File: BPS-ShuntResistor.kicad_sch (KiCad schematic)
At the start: 15 parts, among them J3 Amp_Conn, SW1 SW_DPST

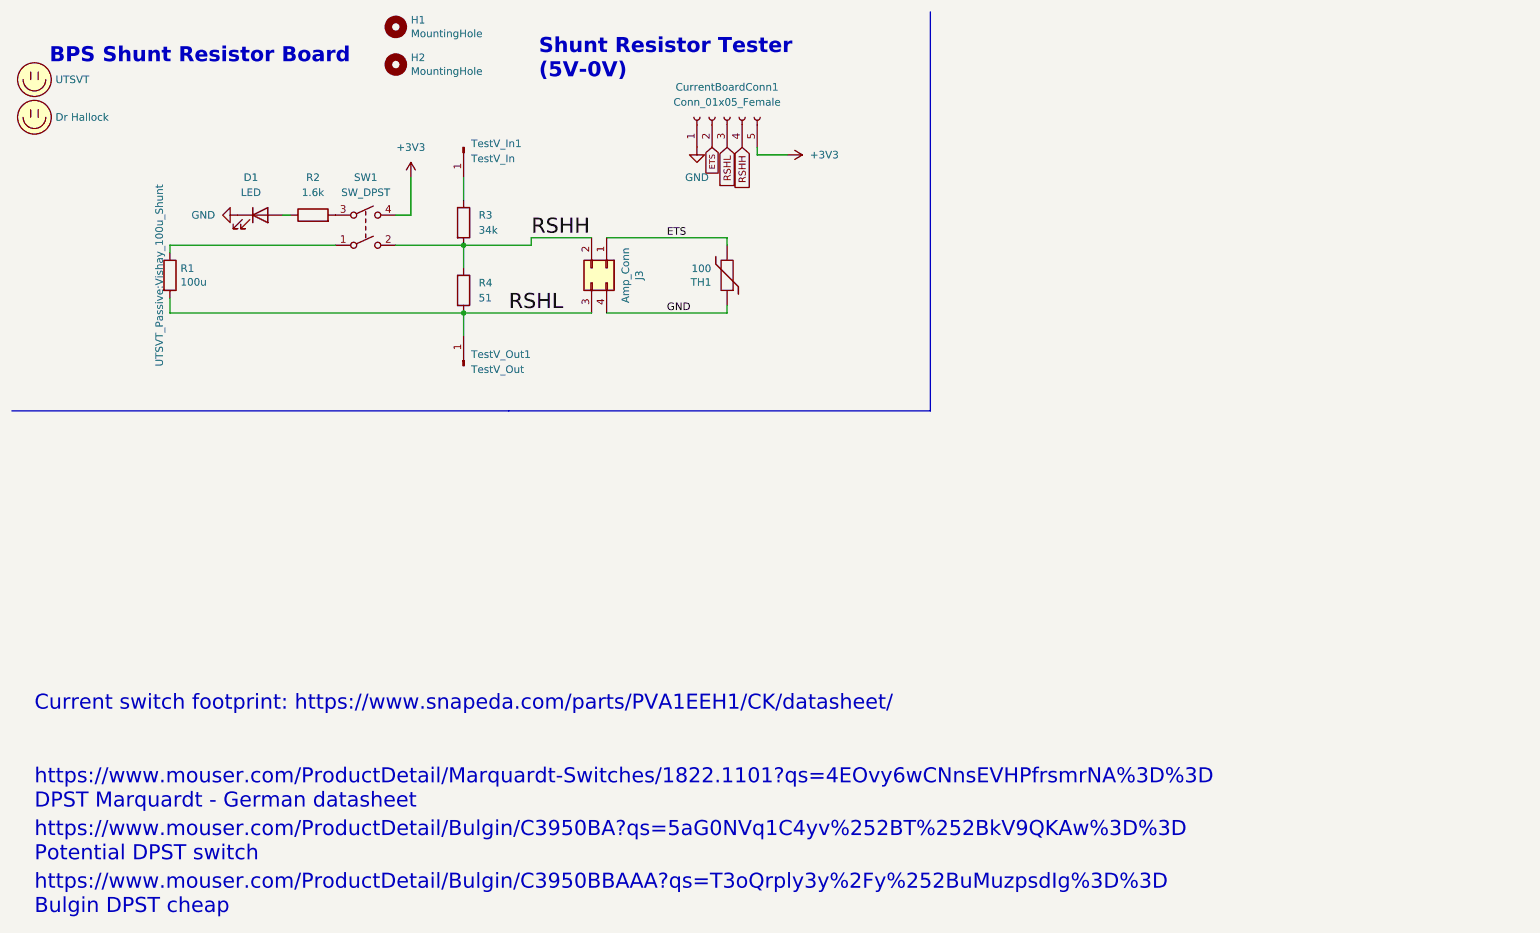
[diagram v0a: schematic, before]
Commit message: added more info per manthan
might need more changes
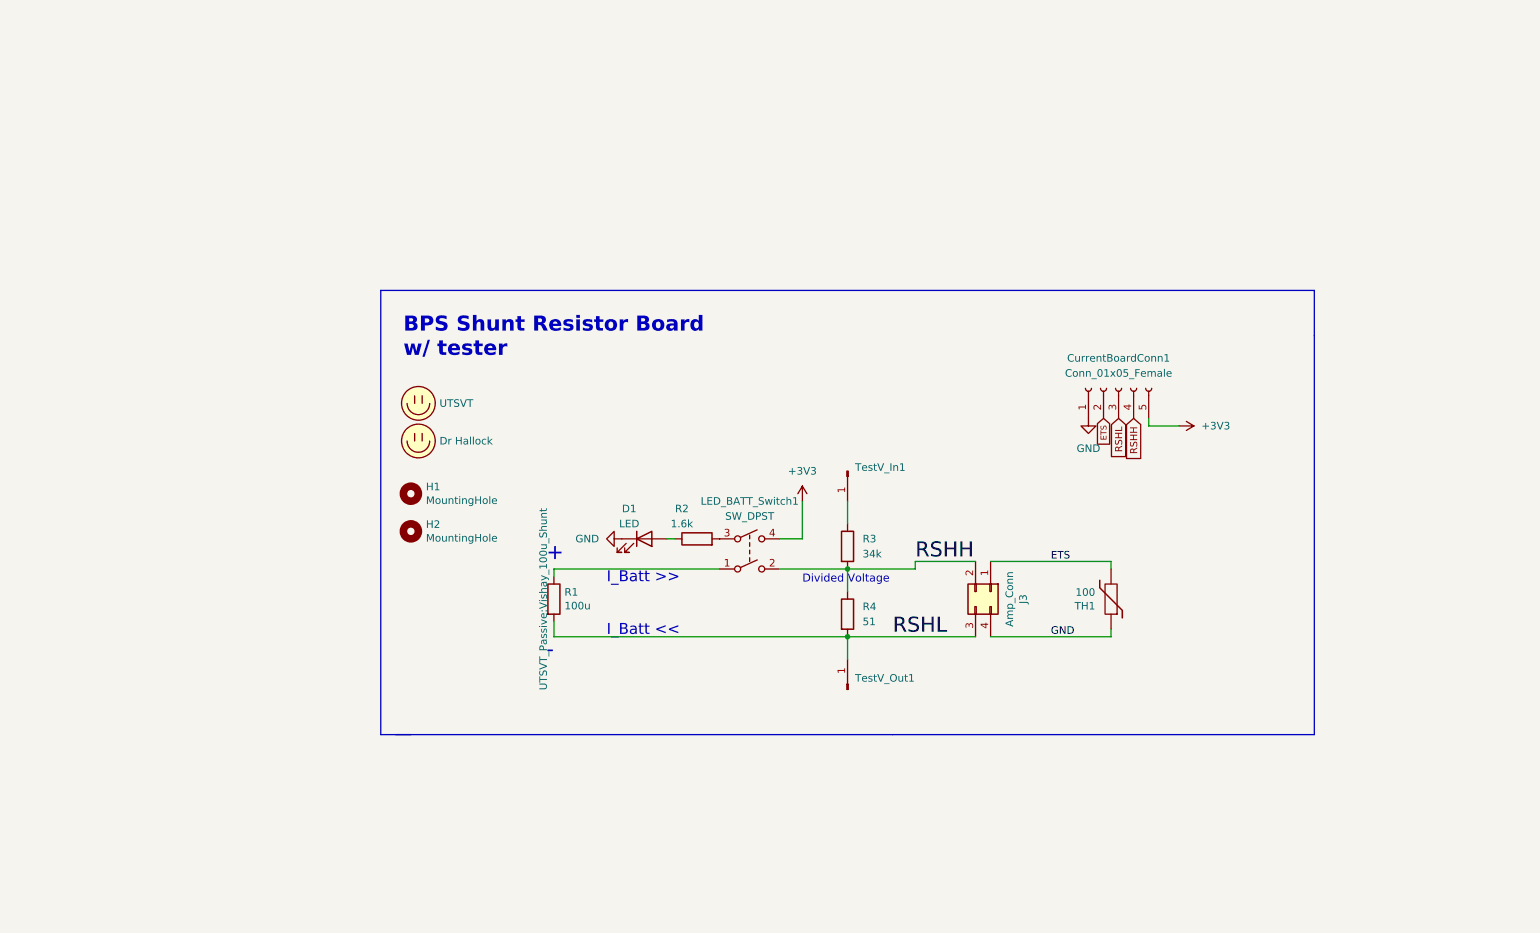
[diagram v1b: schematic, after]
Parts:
- CurrentBoardConn1: footprint Connector_PinSocket_2.54mm:PinSocket_1x05_P2.54mm_Vertical_SMD_Pin1Right -> Connector_PinSocket_2.54mm:PinSocket_1x05_P2.54mm_Vertical
- TestV_In1: value TestV_In -> (none); footprint (none) -> Connector_PinHeader_2.54mm:PinHeader_1x01_P2.54mm_Vertical
- TestV_Out1: value TestV_Out -> (none); footprint (none) -> Connector_PinHeader_2.54mm:PinHeader_1x01_P2.54mm_Vertical
- renumbered SW1 to LED_BATT_Switch1
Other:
- note added: "+ -"
- note added: "BPS Shunt Resistor Board w/ tester"
- note added: "Divided Voltage"
- note added: "I_Batt <<"
- note added: "I_Batt >>"
- note removed: "BPS Shunt Resistor Board"
- note removed: "Current switch footprint: https://www.snapeda.com/parts/PVA1EEH1/CK/datasheet/"
- note removed: "Shunt Resistor Tester (5V-0V)"
- note removed: "https://www.mouser.com/ProductDetail/Bulgin/C3950BA?qs=5aG0NVq1C4yv%252BT%252BkV9QKAw%3D%3D Potential DPST switch"
- note removed: "https://www.mouser.com/ProductDetail/Bulgin/C3950BBAAA?qs=T3oQrply3y%2Fy%252BuMuzpsdIg%3D%3D Bulgin DPST cheap"
- note removed: "https://www.mouser.com/ProductDetail/Marquardt-Switches/1822.1101?qs=4EOvy6wCNnsEVHPfrsmrNA%3D%3D DPST Marquardt - German datasheet"
- moved on the sheet: CurrentBoardConn1, D1, H1, H2, J3, LED_BATT_Switch1, R1, R2, R3, R4, TH1, TestV_In1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
